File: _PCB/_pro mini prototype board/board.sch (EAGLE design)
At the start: 39 parts, among them J2 2p-2.54, J3 2p-2.0, T1_5MM 5mm, T2_5MM 5mm, T3_5MM 5mm

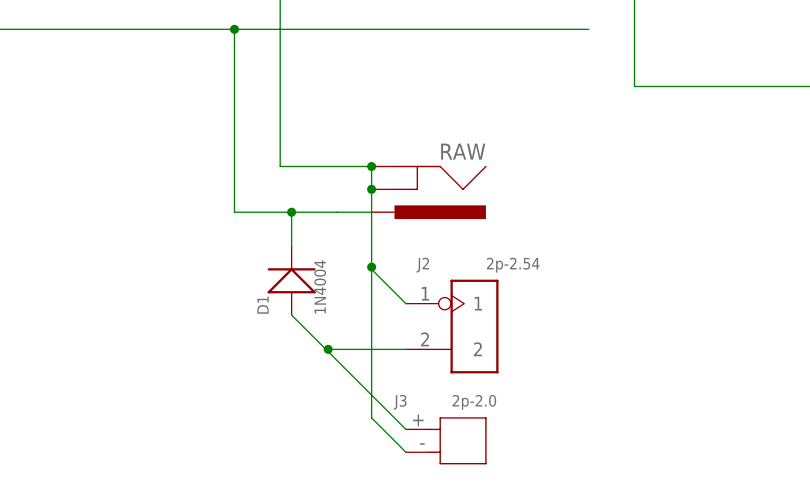
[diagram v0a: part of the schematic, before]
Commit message: PCB optimization
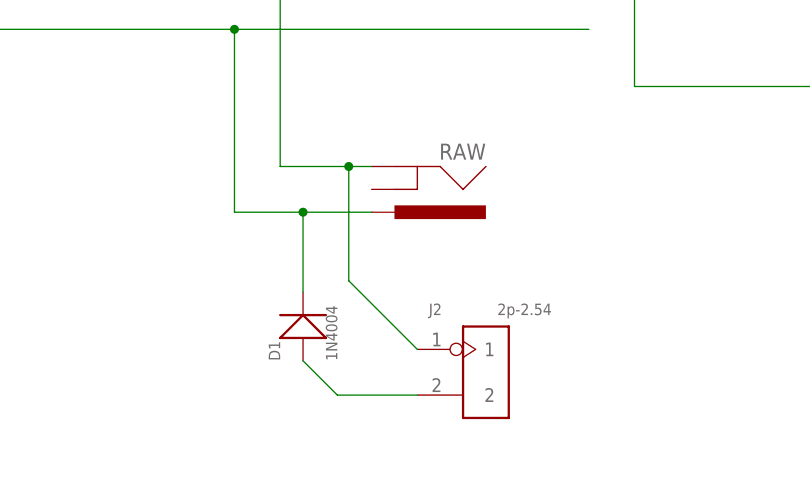
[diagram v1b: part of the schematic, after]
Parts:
- removed J3: 2p-2.0, Seeed-Connector:DIP-JST-2P-2.0
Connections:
- removed net N$28: D1.+, J2.2, J3.P$1
- new net N$24: D1.+, J2.2
- net GND: no longer J3.P$2, RAW.GNDBREAK
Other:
- moved on the sheet: D1, J2
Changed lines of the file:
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@@
 <part name="GND4" library="SparkFun-PowerSymbols" library_urn="urn:adsk.eagle:library:530" deviceset="GND" device=""/>
 <part name="J2" library="Seeed-Connector" library_urn="urn:adsk.eagle:library:478" deviceset="DIP-BLACK-MALE-HEADER-VERT(2P-2.54)" device="" package3d_urn="urn:adsk.eagle:package:33132/1" value="2p-2.54"/>
-<part name="J3" library="Seeed-Connector" library_urn="urn:adsk.eagle:library:478" deviceset="DIP-JST-2P-2.0" device="" package3d_urn="urn:adsk.eagle:package:33112/1" value="2p-2.0"/>
 </parts>
 <sheets>
@@
 <instance part="D13-RAW_1" gate="G$1" x="33.02" y="7.62"/>
 <instance part="D13-RAW_2" gate="G$1" x="53.34" y="7.62"/>
-<instance part="D1" gate="G$1" x="-93.98" y="-53.34" rot="R90"/>
+<instance part="D1" gate="G$1" x="-92.71" y="-58.42" rot="R90"/>
 <instance part="U$1" gate="G$1" x="0" y="7.62"/>
 <instance part="GND1" gate="1" x="-5.08" y="-22.86"/>
 <instance part="GND4" gate="1" x="-17.78" y="35.56"/>
-<instance part="J2" gate="G$1" x="-73.66" y="-58.42"/>
-<instance part="J3" gate="G$1" x="-78.74" y="-71.12"/>
+<instance part="J2" gate="G$1" x="-72.39" y="-63.5"/>
 </instances>
 <busses>
@@
 <label x="-158.75" y="-53.34" size="1.778" layer="95"/>
 <pinref part="RAW" gate="G$1" pin="PWR"/>
-<wire x1="-85.09" y1="-45.72" x2="-88.9" y2="-45.72" width="0.1524" layer="91"/>
-<wire x1="-88.9" y1="-45.72" x2="-93.98" y2="-45.72" width="0.1524" layer="91"/>
-<wire x1="-93.98" y1="-45.72" x2="-100.33" y2="-45.72" width="0.1524" layer="91"/>
+<wire x1="-85.09" y1="-45.72" x2="-92.71" y2="-45.72" width="0.1524" layer="91"/>
+<wire x1="-92.71" y1="-45.72" x2="-100.33" y2="-45.72" width="0.1524" layer="91"/>
 <wire x1="-100.33" y1="-45.72" x2="-100.33" y2="-25.4" width="0.1524" layer="91"/>
 <wire x1="-100.33" y1="-25.4" x2="-60.96" y2="-25.4" width="0.1524" layer="91"/>
 <junction x="-100.33" y="-25.4"/>
 <pinref part="D1" gate="G$1" pin="-"/>
-<wire x1="-93.98" y1="-49.53" x2="-93.98" y2="-45.72" width="0.1524" layer="91"/>
-<junction x="-93.98" y="-45.72"/>
+<wire x1="-92.71" y1="-54.61" x2="-92.71" y2="-45.72" width="0.1524" layer="91"/>
+<junction x="-92.71" y="-45.72"/>
 </segment>
 </net>
@@
 <junction x="-95.25" y="-15.24"/>
 <pinref part="RAW" gate="G$1" pin="GND"/>
-<wire x1="-85.09" y1="-40.64" x2="-95.25" y2="-40.64" width="0.1524" layer="91"/>
+<wire x1="-85.09" y1="-40.64" x2="-87.63" y2="-40.64" width="0.1524" layer="91"/>
+<wire x1="-87.63" y1="-40.64" x2="-95.25" y2="-40.64" width="0.1524" layer="91"/>
 <wire x1="-95.25" y1="-40.64" x2="-95.25" y2="-15.24" width="0.1524" layer="91"/>
 <pinref part="USB_B" gate="G$1" pin="GND"/>
@@
 <junction x="-149.86" y="52.07"/>
 <pinref part="J2" gate="G$1" pin="1"/>
-<wire x1="-81.28" y1="-55.88" x2="-85.09" y2="-52.07" width="0.1524" layer="91"/>
-<wire x1="-85.09" y1="-52.07" x2="-85.09" y2="-51.816" width="0.1524" layer="91"/>
-<junction x="-85.09" y="-40.64"/>
-<pinref part="RAW" gate="G$1" pin="GNDBREAK"/>
-<wire x1="-85.09" y1="-51.816" x2="-85.09" y2="-43.18" width="0.1524" layer="91"/>
-<wire x1="-85.09" y1="-43.18" x2="-85.09" y2="-40.64" width="0.1524" layer="91"/>
-<junction x="-85.09" y="-43.18"/>
-<pinref part="J3" gate="G$1" pin="P$2"/>
-<wire x1="-81.28" y1="-72.39" x2="-85.09" y2="-68.58" width="0.1524" layer="91"/>
-<wire x1="-85.09" y1="-68.58" x2="-85.09" y2="-51.816" width="0.1524" layer="91"/>
-<junction x="-85.09" y="-51.816"/>
+<wire x1="-80.01" y1="-60.96" x2="-87.63" y2="-53.34" width="0.1524" layer="91"/>
+<wire x1="-87.63" y1="-53.34" x2="-87.63" y2="-40.64" width="0.1524" layer="91"/>
+<junction x="-87.63" y="-40.64"/>
 </segment>
 <segment>
@@
 </segment>
 </net>
-<net name="N$28" class="1">
-<segment>
+<net name="N$24" class="0">
+<segment>
+<pinref part="D1" gate="G$1" pin="+"/>
 <pinref part="J2" gate="G$1" pin="2"/>
-<pinref part="D1" gate="G$1" pin="+"/>
-<wire x1="-93.98" y1="-57.15" x2="-90.17" y2="-60.96" width="0.1524" layer="91"/>
-<wire x1="-90.17" y1="-60.96" x2="-89.916" y2="-60.96" width="0.1524" layer="91"/>
-<pinref part="J3" gate="G$1" pin="P$1"/>
-<wire x1="-89.916" y1="-60.96" x2="-81.28" y2="-60.96" width="0.1524" layer="91"/>
-<wire x1="-81.28" y1="-69.85" x2="-89.916" y2="-61.214" width="0.1524" layer="91"/>
-<wire x1="-89.916" y1="-61.214" x2="-89.916" y2="-60.96" width="0.1524" layer="91"/>
-<junction x="-89.916" y="-60.96"/>
-</segment>
-</net>
+<wire x1="-92.71" y1="-62.23" x2="-88.9" y2="-66.04" width="0.1524" layer="91"/>
+<wire x1="-88.9" y1="-66.04" x2="-80.01" y2="-66.04" width="0.1524" layer="91"/>
+</segment>
+</net>
